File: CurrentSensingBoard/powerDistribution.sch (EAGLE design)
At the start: 34 parts, among them J1 XT-60BATT_LABEL, U1 MAX11635EEE+, U2 LM2678SX-5.0/NOPB, U7 AP2114H-3.3TRG1

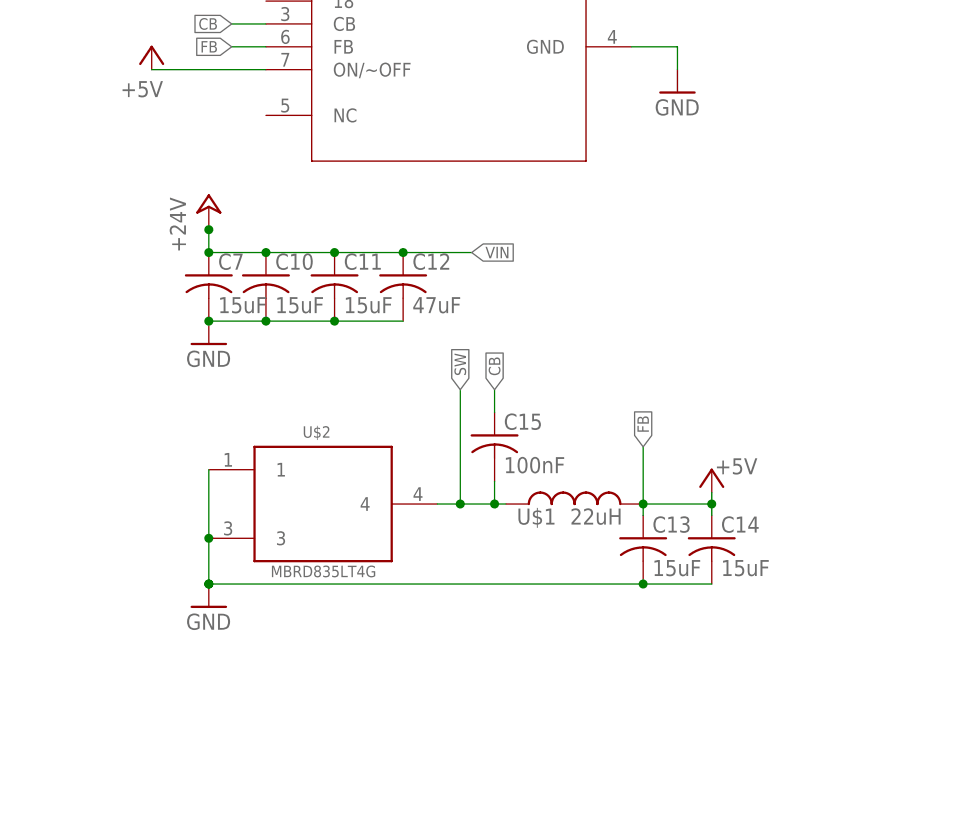
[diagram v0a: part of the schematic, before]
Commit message: added capictors
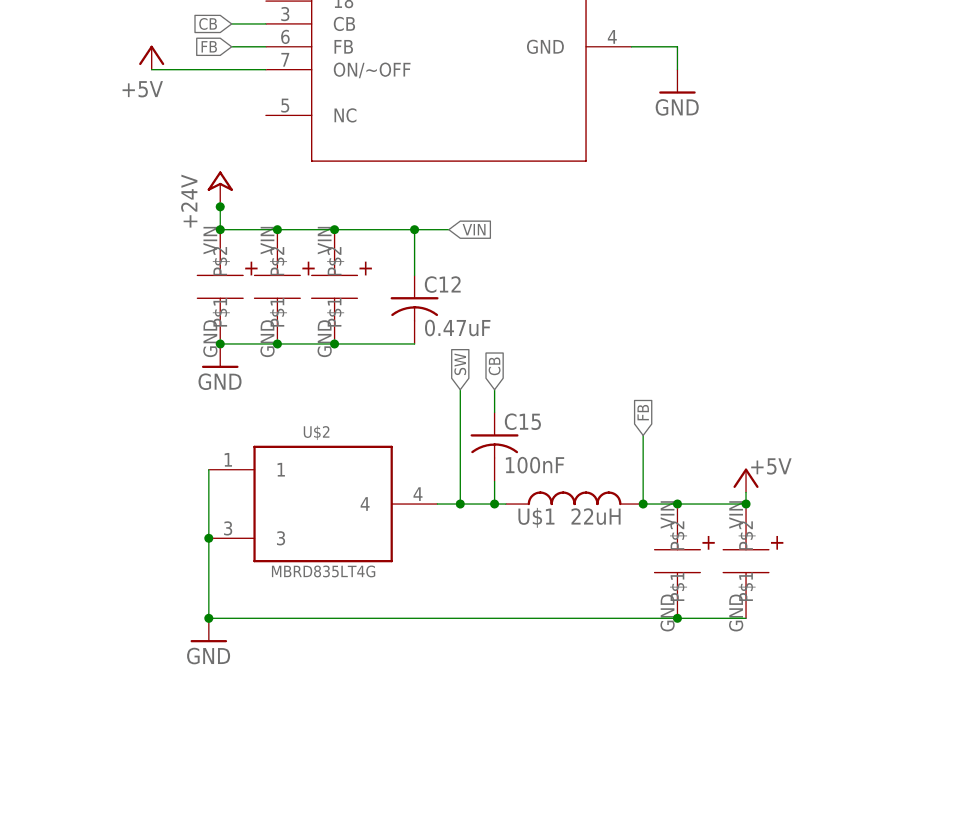
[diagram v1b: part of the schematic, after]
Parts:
- removed C10, C11, C13, C14, C7: 15uF, rcl:C-USC0603
- added U$10, U$8, U$9: 15uF, CurrentSensing:TR3E156M050C0300
- added U$6, U$7: 180uF, CurrentSensing:860010373009
- C12: value 47uF -> 0.47uF
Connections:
- net FB: now also U$6.P$1, U$7.P$1; no longer C13.1, C14.1
- net GND: now also U$10.P$2, U$6.P$2, U$7.P$2, U$8.P$2, U$9.P$2; no longer C10.2, C11.2, C13.2, C14.2, C7.2
- net VIN: now also U$10.P$1, U$8.P$1, U$9.P$1; no longer C10.1, C11.1, C7.1
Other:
- moved on the sheet: C12

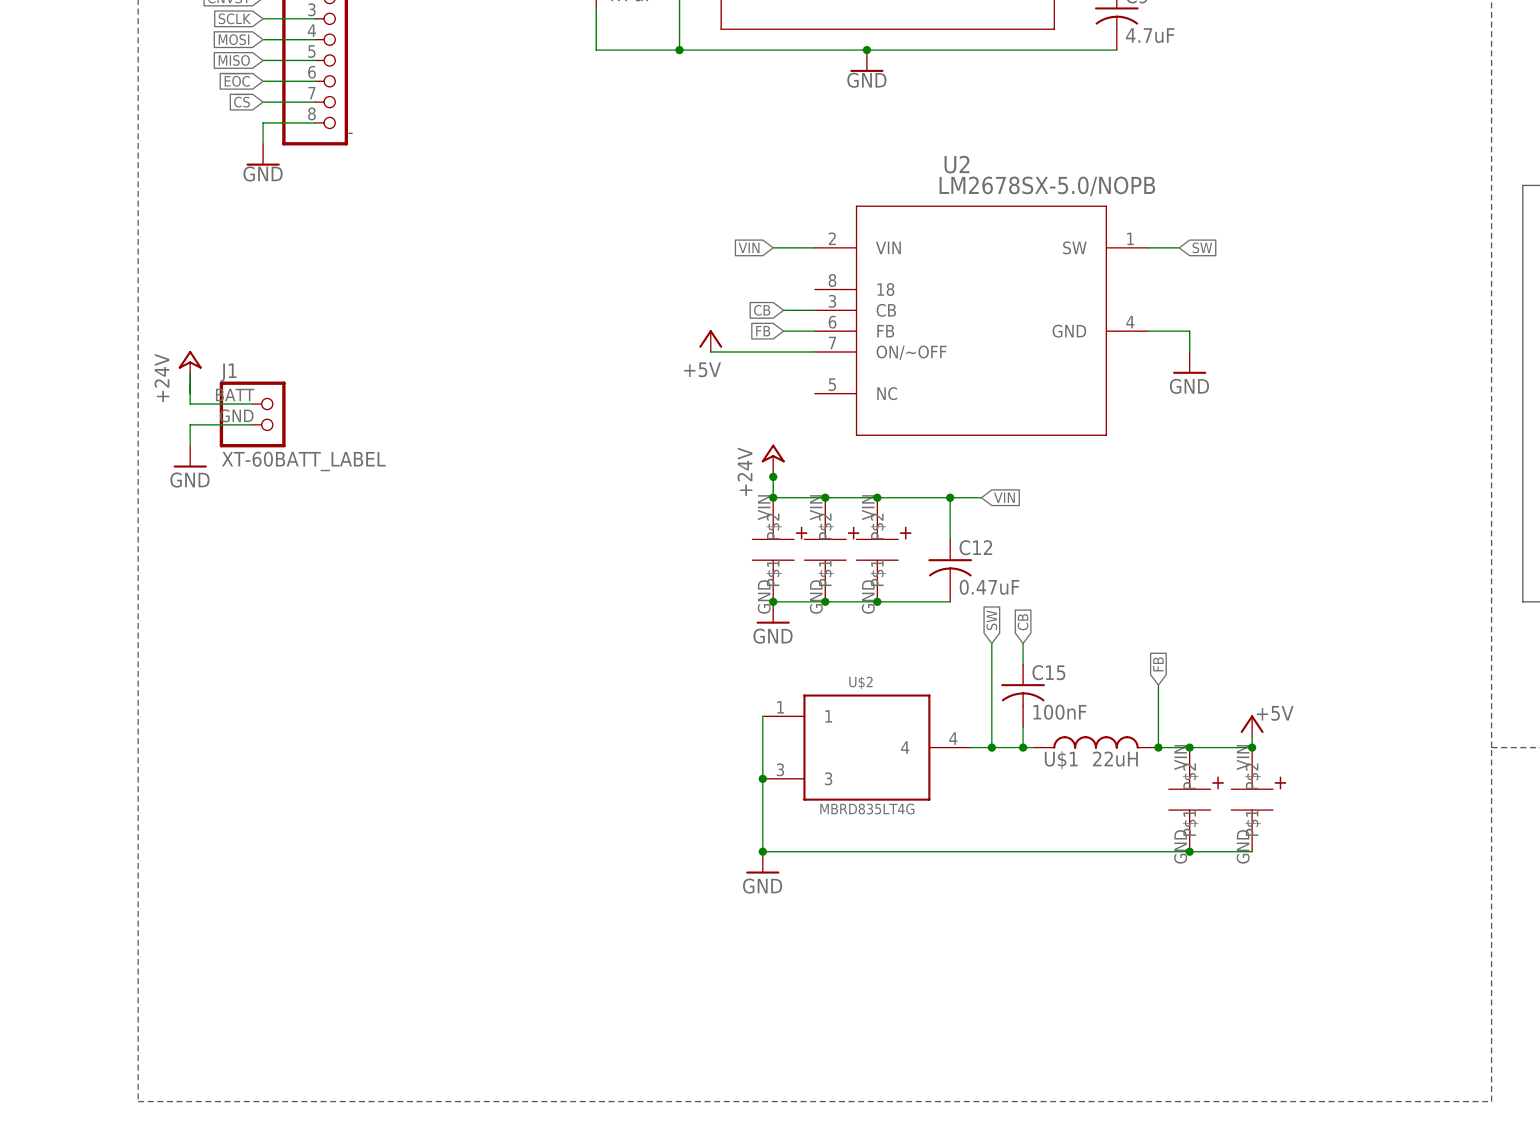
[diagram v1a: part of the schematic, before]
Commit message: fixed Caleb's mess
changed caps and diode symbols
24v regulator footprint was weird
24v regulator schematic looking clean now
deleted unnecessary stuff in library
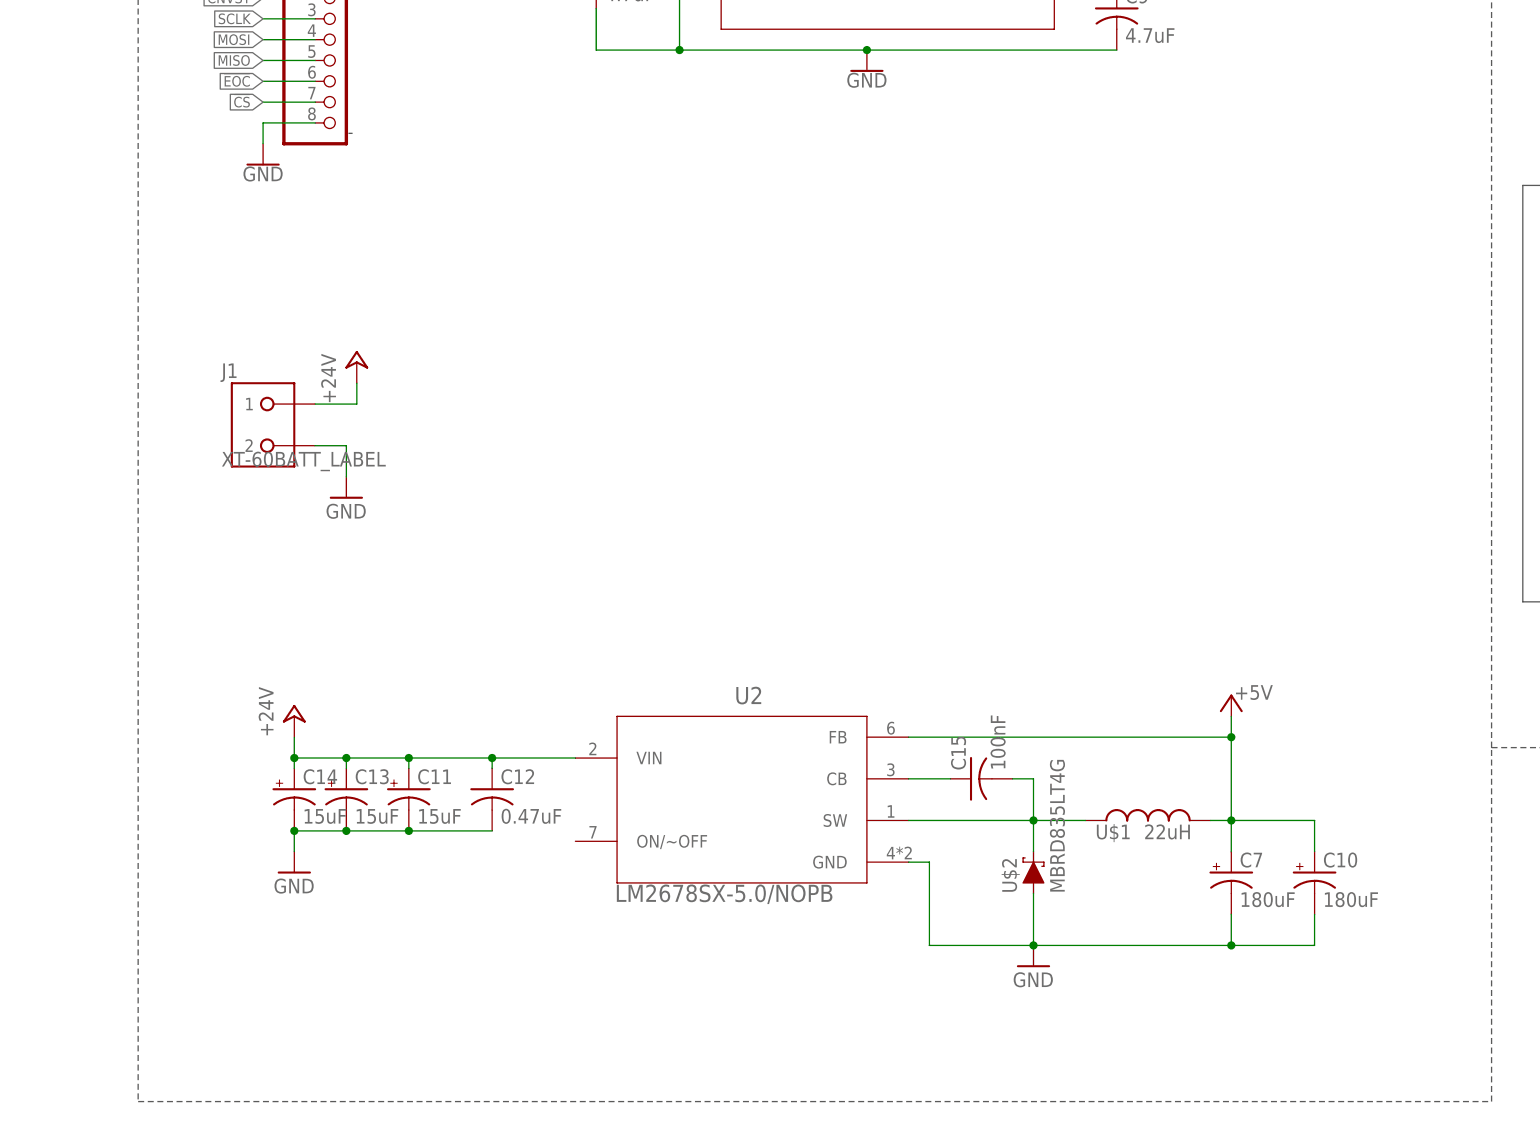
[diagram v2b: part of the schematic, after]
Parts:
- removed U$10, U$8, U$9: 15uF, CurrentSensing:TR3E156M050C0300
- removed U$6, U$7: 180uF, CurrentSensing:860010373009
- added C10, C7: 180uF, CurrentSensing:860010373009
- added C11, C13, C14: 15uF, CurrentSensing:TR3E156M050C0300
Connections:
- net CB renamed N$7
- removed net FB: U$1.2, U$6.P$1, U$7.P$1, U2.FB
- removed net SW: C15.2, U$1.1, U$2.4, U2.SW
- removed net VIN: C12.1, U$10.P$1, U$8.P$1, U$9.P$1, U2.VIN
- new net N$6: C15.2, U$1.1, U$2.C, U2.SW
- net +24V: now also C11.+, C12.1, C13.+, C14.+, U2.VIN
- net +5V: now also C10.+, C7.+, U$1.2, U2.FB; no longer U2.ON/~OFF
- net GND: now also C10.-, C11.-, C13.-, C14.-, C7.-, U$2.A; no longer U$10.P$2, U$2.1, U$2.3, U$6.P$2, U$7.P$2, U$8.P$2, U$9.P$2
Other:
- moved on the sheet: C12, C15, J1, U$1
